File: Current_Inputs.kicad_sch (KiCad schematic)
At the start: 20 parts, among them J6 CURRENT INPUTS, U9 D3V3XA4B10LP

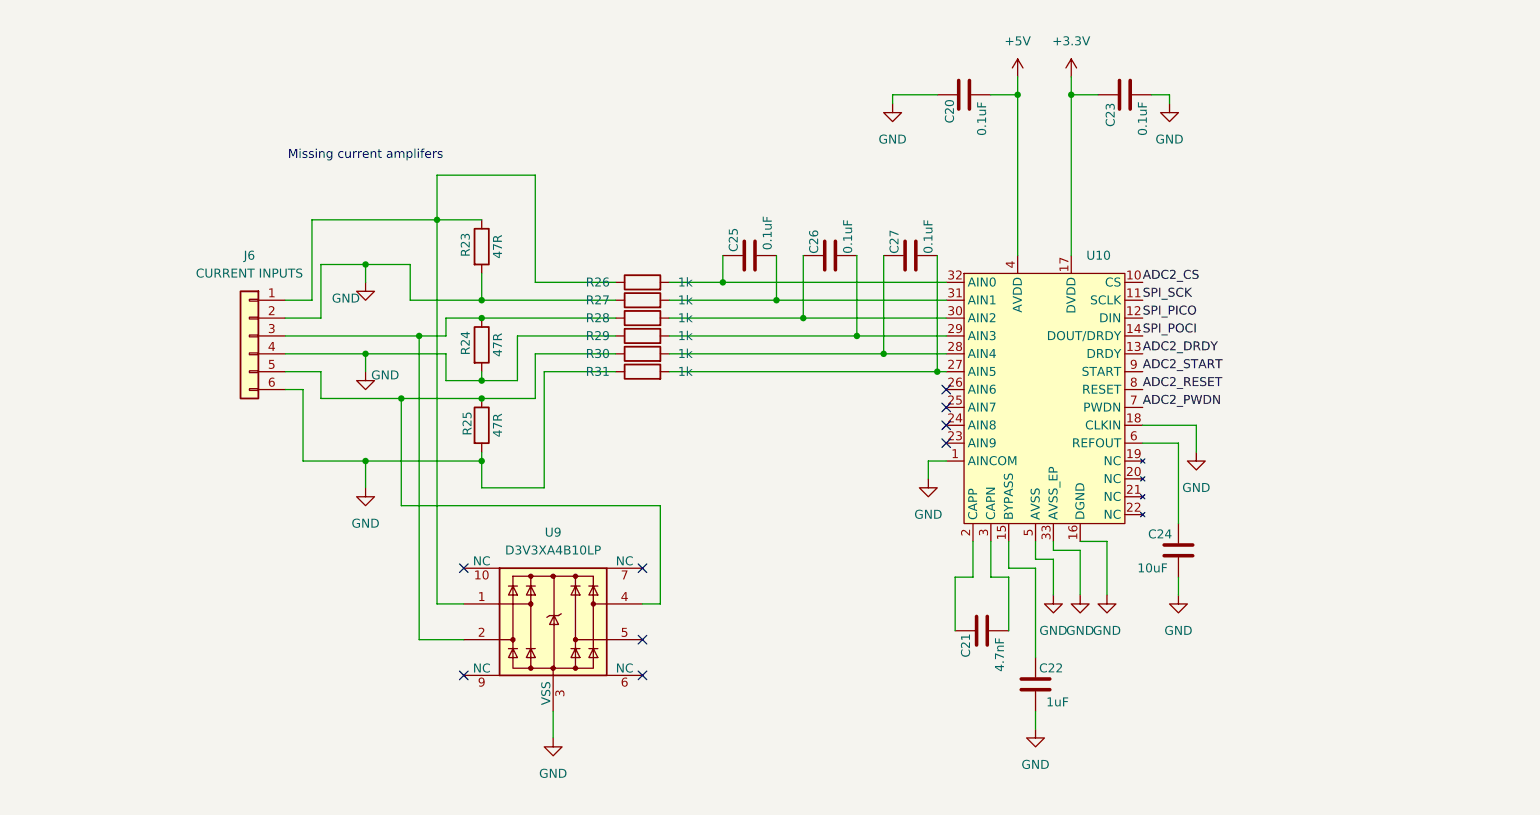
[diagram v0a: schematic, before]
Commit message: finished schematic draft 1
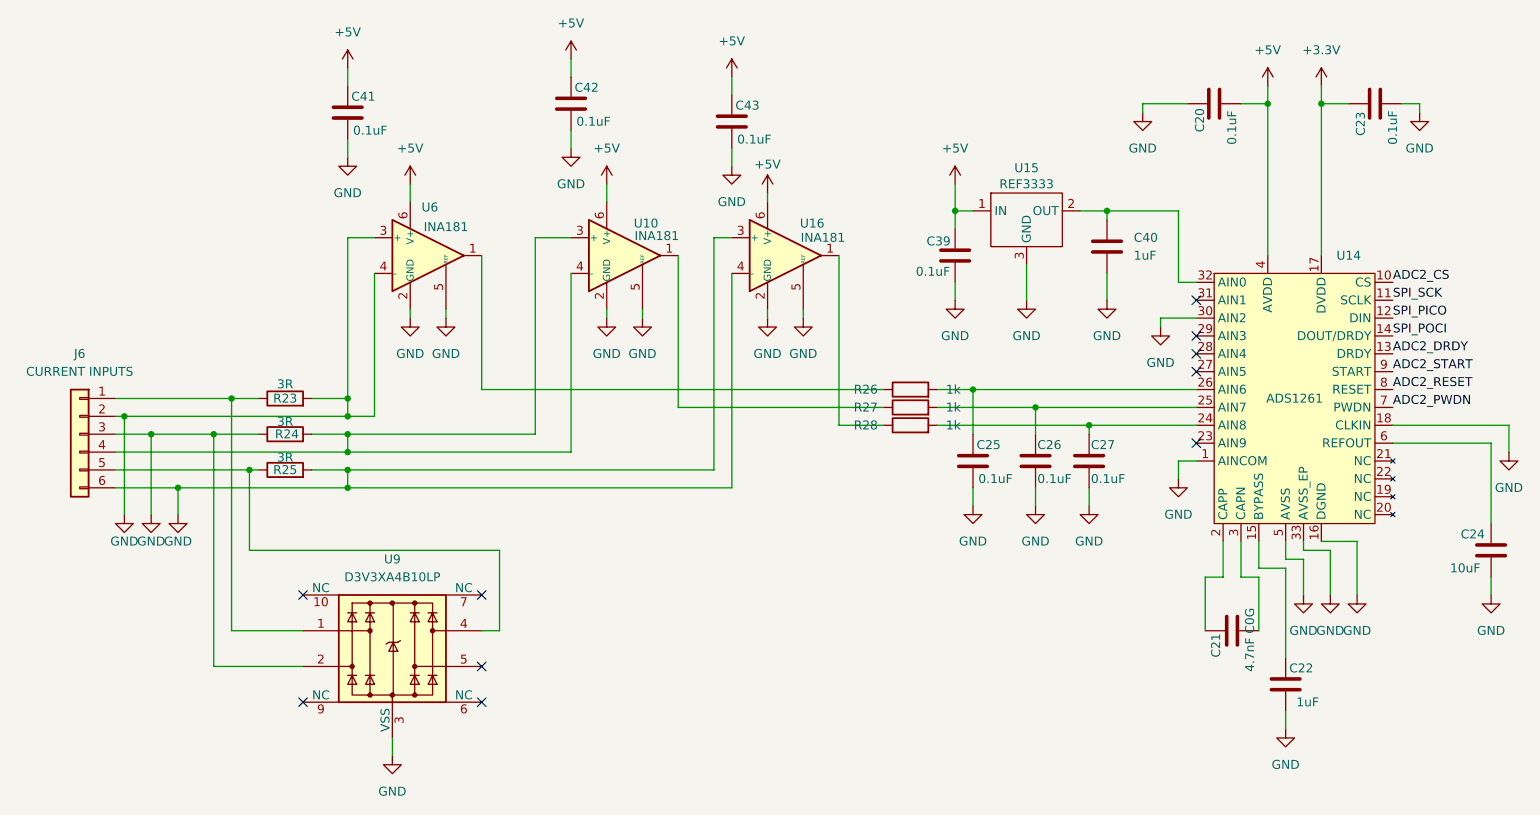
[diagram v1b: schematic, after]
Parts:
- removed R29, R30, R31: 1k, symbol Device:R
- removed U10: (no value), Package_QFP:TQFP-64_10x10mm_P0.5mm, symbol Custom_DT1042-04SO-7:ADS1261
- added C39, C41, C42, C43: 0.1uF, symbol Device:C
- added C40: 1uF, symbol Device:C
- added U10, U16, U6: INA181, Package_TO_SOT_SMD:SOT-23-6, symbol Amplifier_Current:INA181
- added U14: ADS1261, Package_DFN_QFN:QFN-32-1EP_5x5mm_P0.5mm_EP3.45x3.45mm, symbol Custom_ADS1261:ADS1261
- added U15: REF3333, Package_TO_SOT_SMD:SOT-23, symbol Custom_REF3333:REF3333
- C21: value 4.7nF -> 4.7nF C0G
- J6: footprint (none) -> TerminalBlock_Phoenix:TerminalBlock_Phoenix_MKDS-1,5-6-5.08_1x06_P5.08mm_Horizontal; MPN (none) -> 1715763; Manufacturer (none) -> Phoenix Contact
- R23, R24, R25: value 47R -> 3R
- U9: MPN (none) -> D3V3XA4B10LP-7; Manufacturer (none) -> Diodes Incorporated
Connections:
- net +3.3V: now also U14.17 (DVDD)
- net +5V: now also C39.1, C41.1, C42.1, C43.1, U10.6 (V+), U14.4 (AVDD), U15.1 (IN), U16.6 (V+), U6.6 (V+)
- net ADC2_CS: now also U14.10 (CS)
- net ADC2_DRDY: now also U14.13 (DRDY)
- net ADC2_PWDN: now also U14.7 (PWDN)
- net ADC2_RESET: now also U14.8 (RESET)
- net ADC2_START: now also U14.9 (START)
- net GND: now also C25.2, C26.2, C27.2, J6.3 (Pin_3), R24.1, U9.2, C39.2, C40.2, C41.2, C42.2, C43.2, U10.2 (GND), U10.5 (REF), U14.1 (AINCOM), U14.16 (DGND), U14.18 (CLKIN), U14.30 (AIN2), U14.33 (AVSS_EP), U14.5 (AVSS), U15.3 (GND), U16.2 (GND), U16.3 (+), U16.4 (-), U16.5 (REF), U6.2 (GND), U6.3 (+), U6.4 (-), U6.5 (REF); no longer J6.4 (Pin_4), R24.2, R27.1
- net SPI_PICO: now also U14.12 (DIN)
- net SPI_POCI: now also U14.14 (DOUT/DRDY)
- net SPI_SCK: now also U14.11 (SCLK)
- net at C24.1: now also U14.6 (REFOUT)
- net at C22.1: now also U14.15 (BYPASS)
- net at C26.1: now also R27.2, U14.25 (AIN7); no longer R28.2
- net at C27.1: now also R28.2, U14.24 (AIN8)
- net at J6.1 (Pin_1), R23.1, U9.1: no longer R26.1
- net at C21.1: now also U14.2 (CAPP)
- net at C21.2: now also U14.3 (CAPN)
- net at C25.1, R26.2: now also U14.26 (AIN6)
- new net: R27.1, U10.1
- new net: J6.4 (Pin_4), R24.2, U10.3 (+), U10.4 (-)
- new net: C40.1, U14.32 (AIN0), U15.2 (OUT)
- new net: R28.1, U16.1
- new net: R26.1, U6.1
- no-connect marks 9 -> 10
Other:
- note removed: "Missing current amplifers"
- title: Current Inputs -> Current Input
- moved on the sheet: C20, C21, C22, C23, C24, C25, C26, C27, J6, R23, R24, R25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
